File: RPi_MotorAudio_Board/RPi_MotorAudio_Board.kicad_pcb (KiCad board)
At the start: 2 copper layers, 65 x 56 mm, 5 parts, among them P1 Conn_02x20_Odd_Even

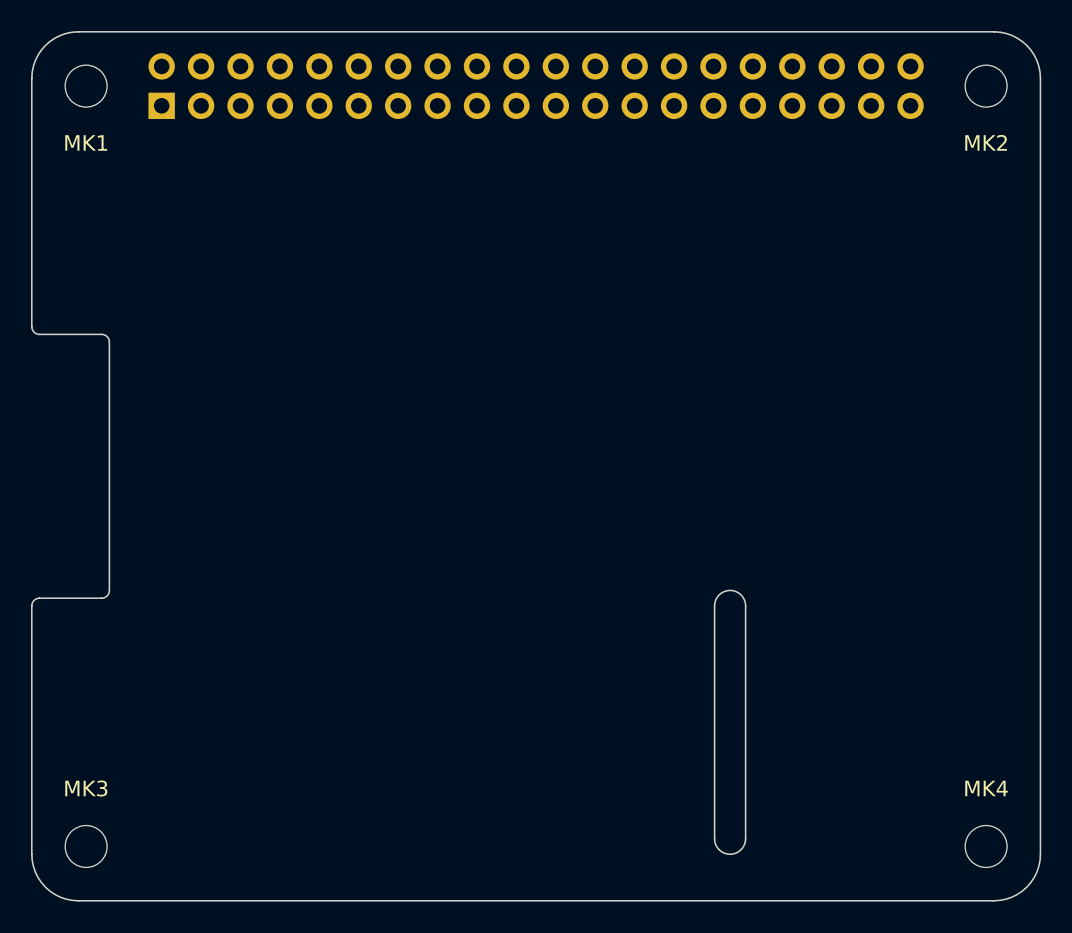
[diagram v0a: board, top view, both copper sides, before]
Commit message: initial layout
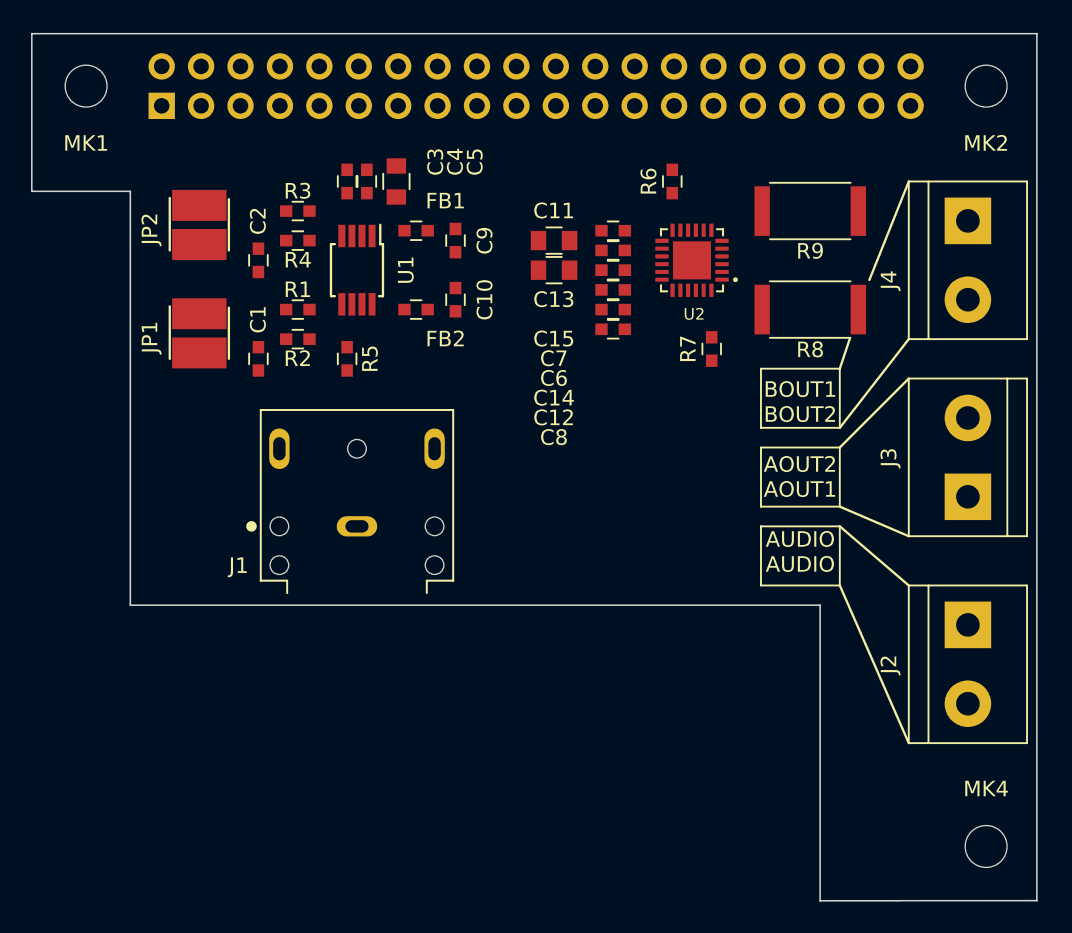
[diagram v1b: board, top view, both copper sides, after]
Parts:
- removed MK3: M2.5, MountingHole:MountingHole_2.7mm_M2.5
- added C1: 0.01uF, Capacitors_SMD:C_0603, F.Cu at (214.6, 115.1)
- added C10: 200pF, Capacitors_SMD:C_0603, F.Cu at (227.3, 111.3)
- added C11: 10uF, Capacitors_SMD:C_0805, F.Cu at (233.7, 107.5)
- added C12: 1uF, Capacitors_SMD:C_0603, F.Cu at (237.5, 111.9)
- added C13: 10uF, Capacitors_SMD:C_0805, F.Cu at (233.7, 109.4)
- added C14: 1uF, Capacitors_SMD:C_0603, F.Cu at (237.5, 110.6)
- added C15: 0.01uF, Capacitors_SMD:C_0603, F.Cu at (237.5, 106.8)
- added C2: 0.01uF, Capacitors_SMD:C_0603, F.Cu at (214.6, 108.7)
- added C3: 1uF, Capacitors_SMD:C_0603, F.Cu at (220.3, 103.6)
- added C4: 1uF, Capacitors_SMD:C_0603, F.Cu at (221.6, 103.6)
- added C5: 10uF, Capacitors_SMD:C_0805, F.Cu at (223.5, 103.6)
- added C6: 0.1uF, Capacitors_SMD:C_0603, F.Cu at (237.5, 109.4)
- added C7: 0.1uF, Capacitors_SMD:C_0603, F.Cu at (237.5, 108.1)
- added C8: 1uF, Capacitors_SMD:C_0603, F.Cu at (237.5, 113.2)
- added C9: 200pF, Capacitors_SMD:C_0603, F.Cu at (227.3, 107.5)
- added FB1: Ferrite_Bead_Small, Capacitors_SMD:C_0603, F.Cu at (224.8, 106.8)
- added FB2: Ferrite_Bead_Small, Capacitors_SMD:C_0603, F.Cu at (224.8, 111.9)
- added J1: SJ1-3523N, KiCad_Offline:CUI_SJ1-3523N, F.Cu at (221.0, 125.9)
- added J2: SPEAKER, Connectors_Terminal_Blocks:TerminalBlock_bornier-2_P5.08mm, F.Cu at (260.3, 132.2)
- added J3: STEP_1, Connectors_Terminal_Blocks:TerminalBlock_bornier-2_P5.08mm, F.Cu at (260.3, 124.0)
- added J4: STEP_2, Connectors_Terminal_Blocks:TerminalBlock_bornier-2_P5.08mm, F.Cu at (260.3, 106.2)
- added JP1: SolderJumper_2_Open, UserFootprints:Inductor_SMD_3.0mm_x_3.0mm, F.Cu at (210.8, 113.2)
- added JP2: SolderJumper_2_Open, UserFootprints:Inductor_SMD_3.0mm_x_3.0mm, F.Cu at (210.8, 106.2)
- added R1: 150k, Capacitors_SMD:C_0603, F.Cu at (217.1, 111.9)
- added R2: 150k, Capacitors_SMD:C_0603, F.Cu at (217.1, 113.8)
- added R3: 150k, Capacitors_SMD:C_0603, F.Cu at (217.1, 105.5)
- added R4: 150k, Capacitors_SMD:C_0603, F.Cu at (217.1, 107.5)
- added R5: 51k, Capacitors_SMD:C_0603, F.Cu at (220.3, 115.1)
- added R6: 51k, Capacitors_SMD:C_0603, F.Cu at (241.3, 103.6)
- added R7: 51k, Capacitors_SMD:C_0603, F.Cu at (243.8, 114.4)
- added R8: 0.5, Resistors_SMD:R_2512, F.Cu at (250.2, 111.9)
- added R9: 0.5, Resistors_SMD:R_2512, F.Cu at (250.2, 105.5)
- added U1: PAM8303AAD, Housings_SSOP:MSOP-8_3x3mm_Pitch0.65mm, F.Cu at (221.0, 109.4)
- added U2: DRV8834-VQFN, KiCad_Offline:QFN50P400X400X100-25N, F.Cu at (242.5, 108.7)
- MK1, MK2, MK4: footprint MountingHole:MountingHole_2.7mm_M2.5 -> Mounting_Holes:MountingHole_2.7mm_M2.5
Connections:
- net /GPIO10(SPI0_MOSI) renamed Net-(P1-Pad19)
- net /GPIO11(SPI0_SCK) renamed Net-(P1-Pad23)
- net /GPIO14(TXD0) renamed Net-(P1-Pad8)
- net /GPIO15(RXD0) renamed Net-(P1-Pad10)
- net /GPIO17(GEN0) renamed Net-(P1-Pad11)
- net /GPIO18(GEN1)(PWM0) renamed Net-(P1-Pad12)
- net /GPIO2(SDA1) renamed Net-(P1-Pad3)
- net /GPIO20(SPI1_MOSI) renamed Net-(P1-Pad38)
- net /GPIO21(SPI1_SCK) renamed Net-(P1-Pad40)
- net /GPIO22(GEN3) renamed Net-(P1-Pad15)
- net /GPIO23(GEN4) renamed Net-(P1-Pad16)
- net /GPIO24(GEN5) renamed Net-(P1-Pad18)
- net /GPIO25(GEN6) renamed Net-(P1-Pad22)
- net /GPIO27(GEN2) renamed Net-(P1-Pad13)
- net /GPIO3(SCL1) renamed Net-(P1-Pad5)
- net /GPIO4(GCLK) renamed Net-(P1-Pad7)
- net /GPIO7(SPI1_CE_N) renamed Net-(P1-Pad26)
- net /GPIO8(SPI0_CE_N) renamed Net-(P1-Pad24)
- net /GPIO9(SPI0_MISO) renamed Net-(P1-Pad21)
- net /ID_SC renamed Net-(P1-Pad28)
- net /ID_SD renamed Net-(P1-Pad27)
- P1 pad 29: /GPIO5 -> /GPIO5_DIR
- P1 pad 31: /GPIO6 -> /GPIO6_M0
- P1 pad 32: /GPIO12(PWM0) -> /GPIO12(PWM0)_STEP
- P1 pad 33: /GPIO13(PWM1) -> /GPIO13_M1
- P1 pad 35: /GPIO19(SPI1_MISO) -> /GPIO19_~SLEEP
- P1 pad 36: /GPIO16 -> /GPIO16_~FAULT
- P1 pad 37: /GPIO26 -> /GPIO26_DECAY
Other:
- board size 65 x 56 mm -> 64.8 x 55.9 mm
- board text added: "BOUT1 BOUT2 AOUT2 AOUT1 AUDIO AUDIO"
- board text removed: "CAMERA"
- board text removed: "DISPLAY"
